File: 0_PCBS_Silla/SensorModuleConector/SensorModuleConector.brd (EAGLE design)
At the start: 29.2 x 40 mm, 11 parts

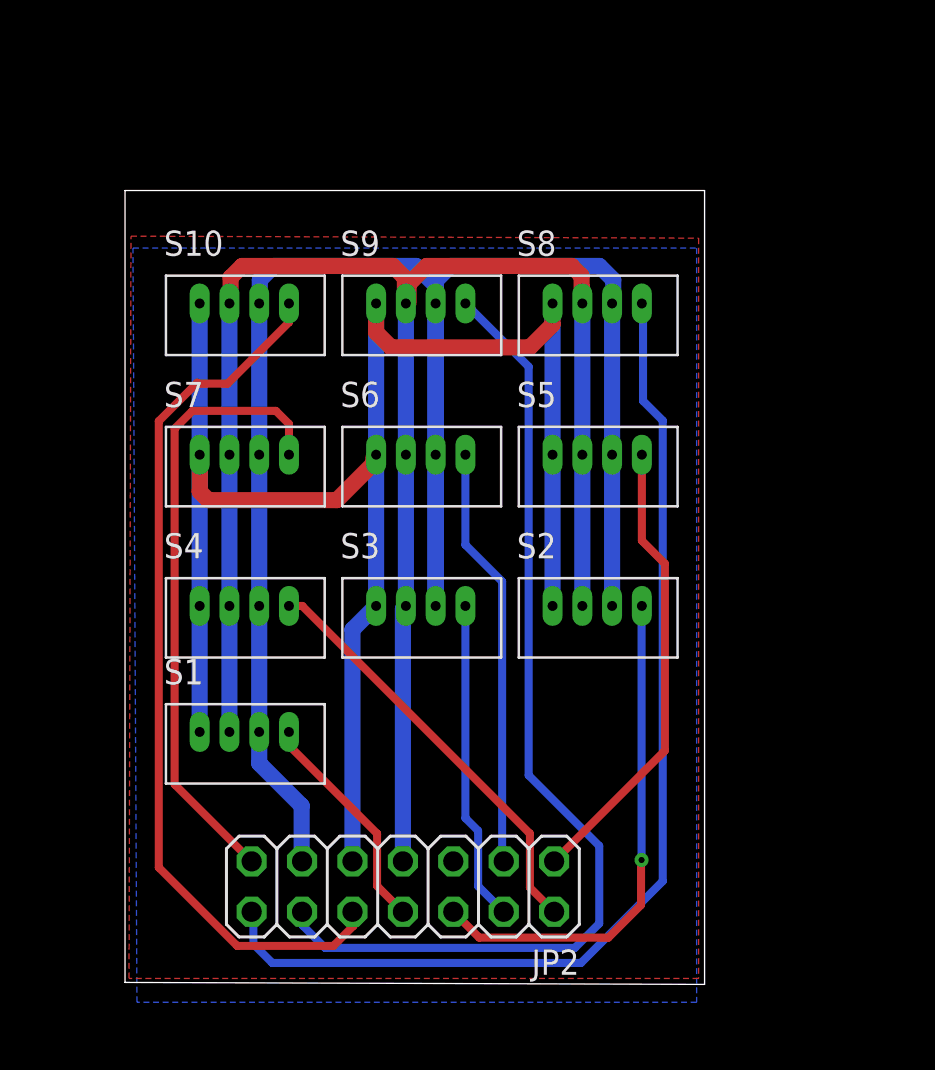
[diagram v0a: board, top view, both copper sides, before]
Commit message: 20 marzo 2020
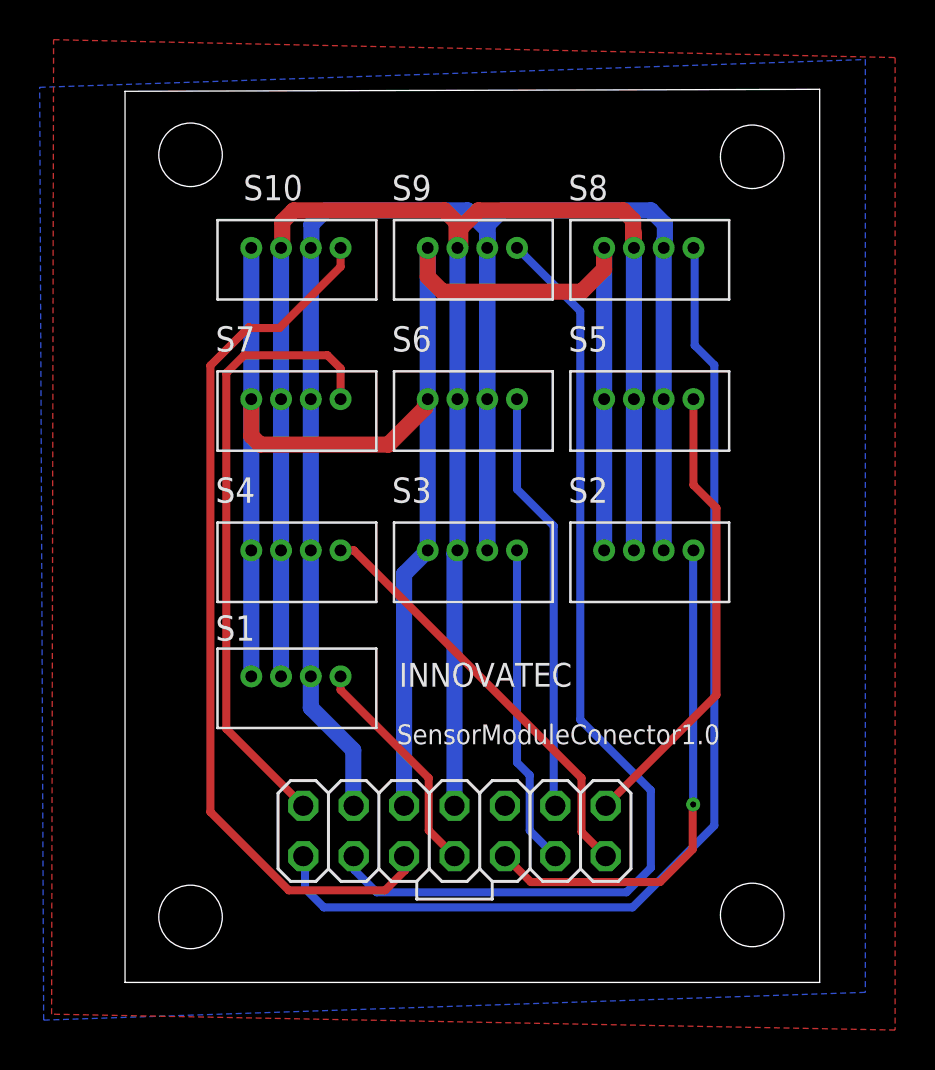
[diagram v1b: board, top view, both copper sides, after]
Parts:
- moved S2 3.82 mm to (26.3, 21.8)
- moved S5 3.82 mm to (26.3, 29.4)
- moved JP2 3.82 mm to (16.6, 7.63)
- moved S1 3.82 mm to (8.56, 15.4)
- moved S4 3.82 mm to (8.56, 21.8)
- moved S7 3.82 mm to (8.56, 29.4)
- moved S3 3.82 mm to (17.4, 21.8)
- moved S6 3.82 mm to (17.4, 29.4)
- moved S8 3.82 mm to (26.3, 37.0)
- moved S10 3.82 mm to (8.56, 37.0)
- moved S9 3.82 mm to (17.4, 37.0)
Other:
- board size 29.2 x 40 mm -> 35 x 45 mm
- board text added: "INNOVATEC"
- board text added: "SensorModuleConector1.0"
